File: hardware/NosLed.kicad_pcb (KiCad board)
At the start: 2 copper layers, 127 x 118.1 mm, 40 parts, among them J101 AC, J102 PWM, J103 380OUT, J104 380_BP2876D, J105 LOAD, J107 3V3, J108 380_LNK302PN, U301 BP2876, U401 AMS1117-3.3, U402 LNK306P

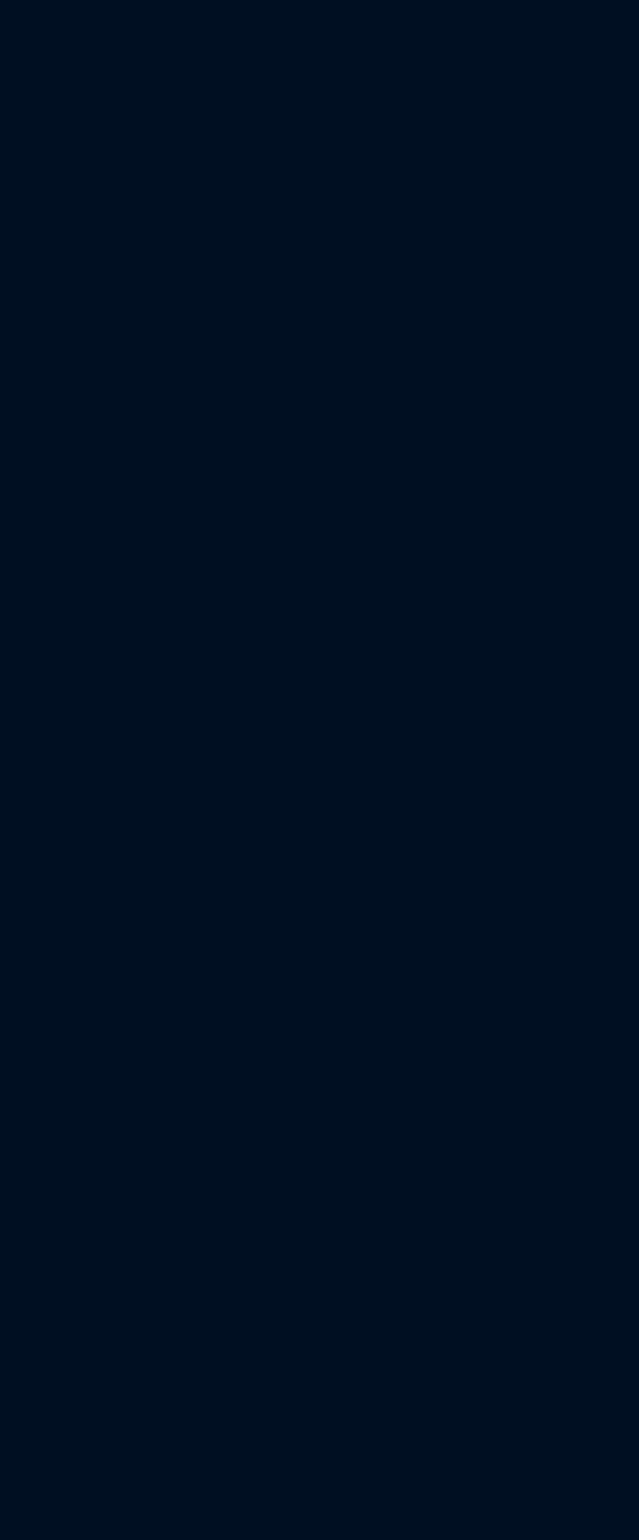
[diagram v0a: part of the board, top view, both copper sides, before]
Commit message: BP2956XS
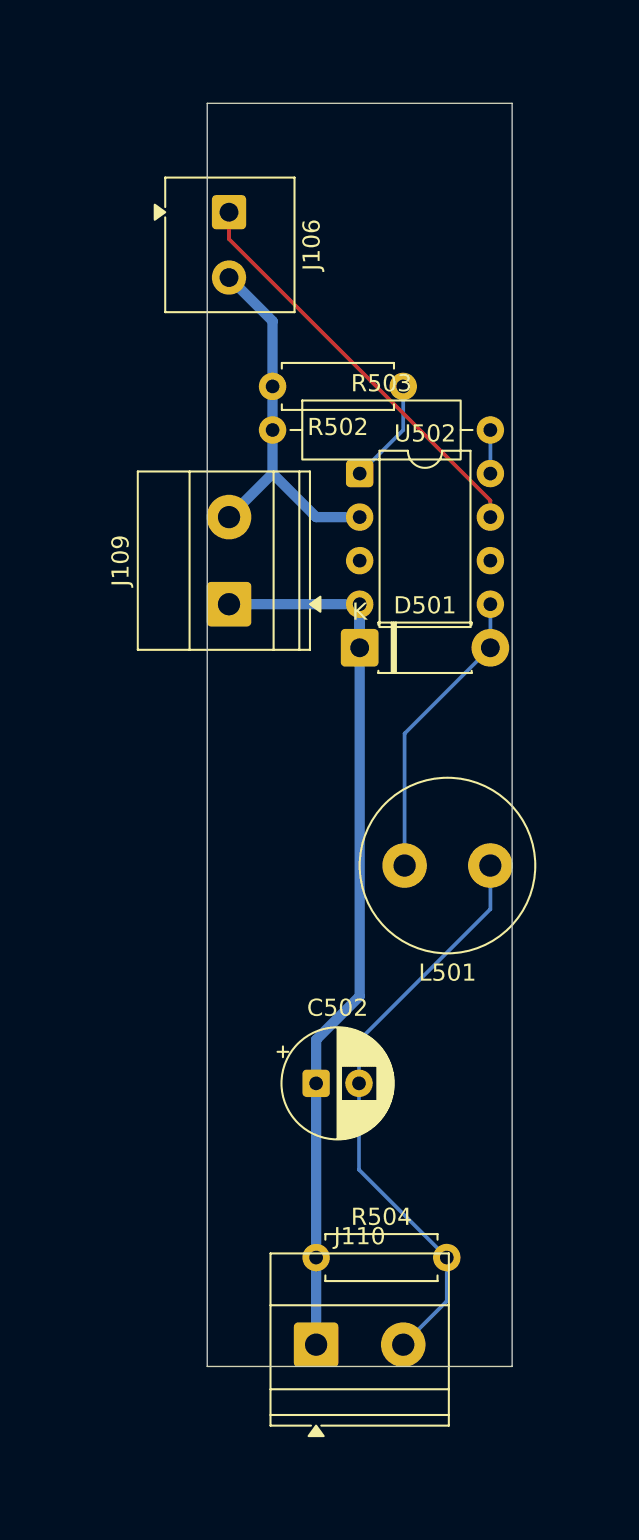
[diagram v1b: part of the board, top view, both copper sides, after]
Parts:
- added C502: 10uF 100v, Capacitor_THT:CP_Radial_D6.3mm_P2.50mm, F.Cu at (114.3, 81.3)
- added D501: UF4007, Diode_THT:D_DO-41_SOD81_P7.62mm_Horizontal, F.Cu at (116.8, 55.9)
- added J106: PWM1, TerminalBlock_Phoenix:TerminalBlock_Phoenix_MKDS-1-2-3.81_1x02_P3.81mm_Horizontal, F.Cu at (109.2, 30.5)
- added J109: 380_BP2956XS, TerminalBlock_Phoenix:TerminalBlock_Phoenix_MKDS-1,5-2-5.08_1x02_P5.08mm_Horizontal, F.Cu at (109.2, 53.3)
- added J110: LOAD2, TerminalBlock_Phoenix:TerminalBlock_Phoenix_MKDS-1,5-2-5.08_1x02_P5.08mm_Horizontal, F.Cu at (114.3, 96.5)
- added L501: 2.2mH, Inductor_THT:L_Radial_D10.0mm_P5.00mm_Fastron_07M, F.Cu at (124.5, 68.6)
- added R502: 7K5, Resistor_THT:R_Axial_DIN0207_L6.3mm_D2.5mm_P7.62mm_Horizontal, F.Cu at (119.4, 40.6)
- added R503: 2R7, Resistor_THT:R_Axial_DIN0309_L9.0mm_D3.2mm_P12.70mm_Horizontal, F.Cu at (111.8, 43.2)
- added R504: 100К, Resistor_THT:R_Axial_DIN0207_L6.3mm_D2.5mm_P7.62mm_Horizontal, F.Cu at (114.3, 91.4)
- added U502: BP2956XS, Package_DIP:DIP-8_W7.62mm, F.Cu at (116.8, 45.7)
- C202, C203: value 22uF 400v -> 15uF 400v
- C406: value 22uF 10V -> 100uF 10V
- D401: value ES1J (UF4007) -> ES1J
- D402: value 1N4007 -> US1M
- J102: value PWM -> PWM2
- J105: value LOAD -> LOAD2
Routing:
- net /ACInput/380V: track 67.8 -> 122.2 mm
- net /BP2956XS/LOAD-: track 0.00 -> 34.3 mm
- net /BP2956XS/PWM: track 0.00 -> 24.1 mm
- net /BP2876D/PWR_GND: track 150.7 -> 172.9 mm
- net /BP2956XS/DRAIN: track 0.00 -> 17.3 mm
- net Net-(U502-ROVP): track 0.00 -> 6.13 mm
- net /BP2956XS/CS: track 0.00 -> 2.54 mm
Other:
- outline, holes or cut-outs redrawn
